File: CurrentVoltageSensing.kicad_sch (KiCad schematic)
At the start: 9 parts, among them U1 TMCS1170

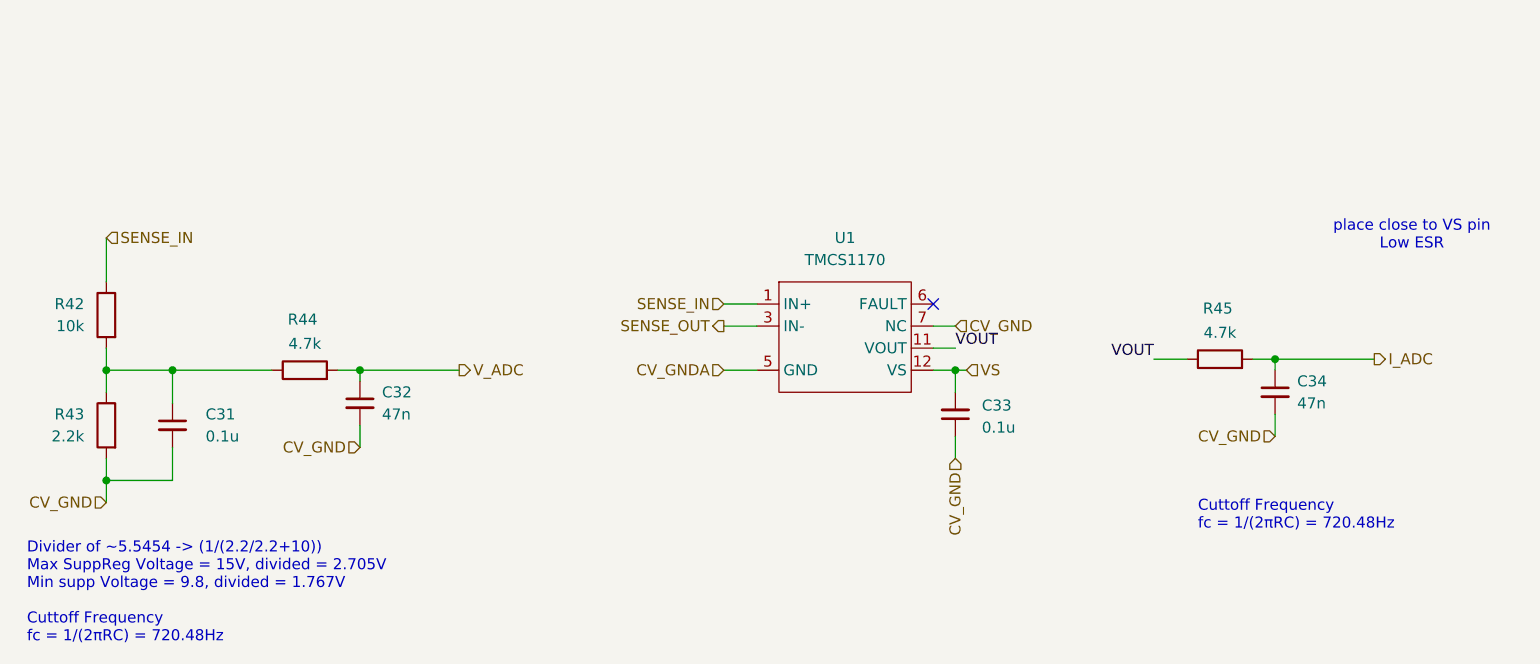
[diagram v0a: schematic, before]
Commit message: newcvsense
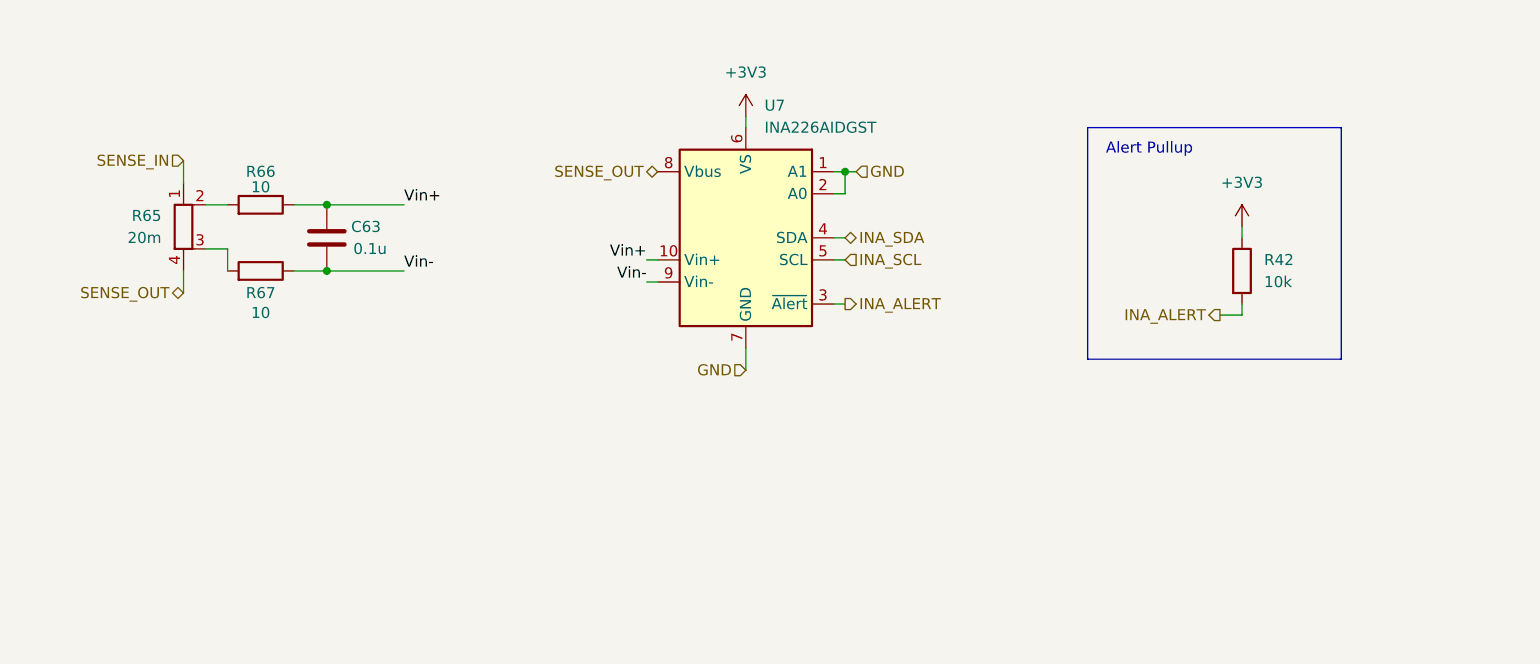
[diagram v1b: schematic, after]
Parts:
- removed C31, C33: 0.1u, Capacitor_SMD:C_0603_1608Metric_Pad1.08x0.95mm_HandSolder, symbol Device:C_Small
- removed C32, C34: 47n, Capacitor_SMD:C_0603_1608Metric_Pad1.08x0.95mm_HandSolder, symbol Device:C_Small
- removed R43: 2.2k, Resistor_SMD:R_0603_1608Metric_Pad0.98x0.95mm_HandSolder, symbol Device:R
- removed R44, R45: 4.7k, Resistor_SMD:R_0603_1608Metric_Pad0.98x0.95mm_HandSolder, symbol Device:R
- removed U1: TMCS1170, symbol PS-SuppCharger_Library:TMCS1170
- added C63: 0.1u, symbol Device:C
- added R65: 20m, symbol Device:R_Shunt
- added R66, R67: 10, symbol Device:R
- added U7: INA226AIDGST, Package_SO:TSSOP-10_3x3mm_P0.5mm, symbol Sensor_Energy:INA226
- R42: footprint Resistor_SMD:R_0603_1608Metric_Pad0.98x0.95mm_HandSolder -> (none); Assemble -- mixed values -- -> (none); LCSC P/N C25804 -> (none); Mouser Part Number -- mixed values -- -> (none); P/N -- mixed values -- -> (none)
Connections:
- net SENSE_IN: now also R65.1; no longer R42.1
- net SENSE_OUT: now also R65.4, U7.8 (Vbus)
- net INA_ALERT: now reaches R42.2
- net INA_ALERT: now also U7.3 (~{Alert})
- new net: R65.2, R66.2
- new net: R65.3, R67.2
- new net +3V3: R42.1, U7.6 (VS)
- new net GND: U7.1 (A1), U7.2 (A0), U7.7 (GND)
- new net INA_SCL: U7.5 (SCL)
- new net INA_SDA: U7.4 (SDA)
- new net Vin+: C63.1, R66.1, U7.10 (Vin+)
- new net Vin-: C63.2, R67.1, U7.9 (Vin-)
- no-connect marks 1 -> 0
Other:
- note added: "Alert Pullup"
- note removed: "Cuttoff Frequency fc = 1/(2πRC) = 720.48Hz"
- note removed: "Divider of ~5.5454 -> (1/(2.2/2.2+10)) Max SuppReg Voltage = 15V, divided = 2.705V Min supp Voltage = 9.8, divided = 1.767V Cuttoff Frequency fc = 1/(2πRC) = 720.48Hz"
- note removed: "place close to VS pin Low ESR"

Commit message: shuntschem2
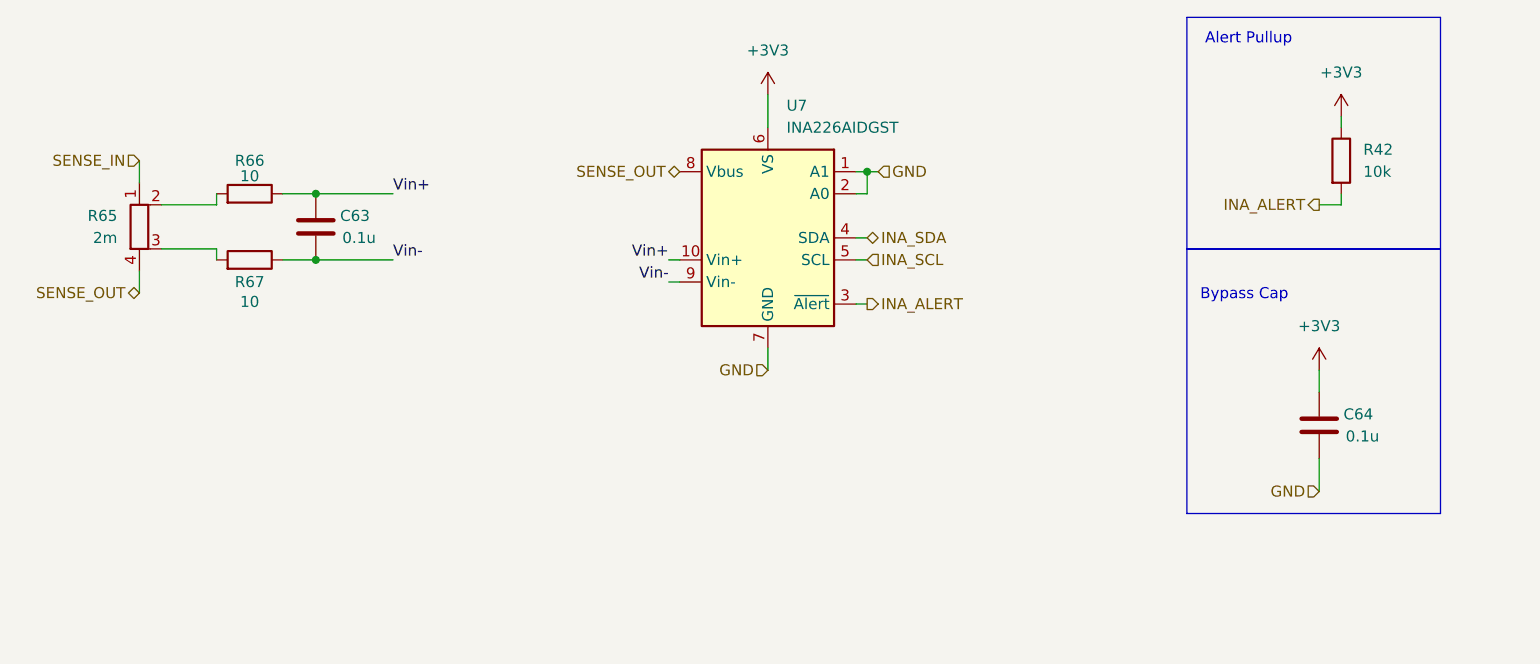
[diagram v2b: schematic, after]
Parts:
- added C64: 0.1u, symbol Device:C
- R65: value 20m -> 2m
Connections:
- net +3V3: now also C64.1
- net GND: now also C64.2
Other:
- note added: "Bypass Cap"
- moved on the sheet: C63, R42, R65, R66, R67, U7
